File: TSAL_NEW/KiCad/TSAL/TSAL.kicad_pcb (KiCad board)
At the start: 2 copper layers, 74.8 x 40.6 mm, 34 parts, among them J1 HV INPUT, J2 HV GND, J3 Pin Storage, J4 Green_LED_Jp, J5 Conn_02x02_Counter_Clockwise, Q1 BSS84, Q2 BSS84, U1 LTV-817S, U2 LR8K4-G, U4 LM555

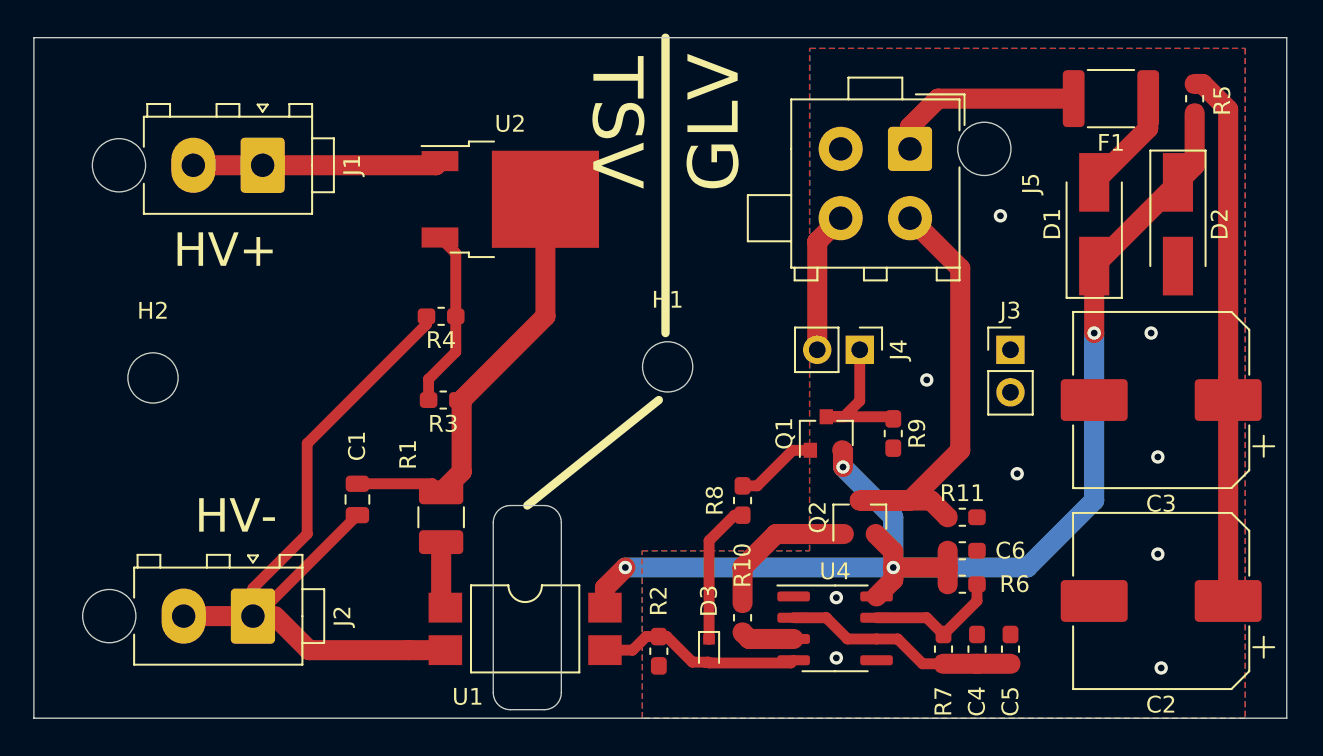
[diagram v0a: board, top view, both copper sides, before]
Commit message: TSAL Review complete
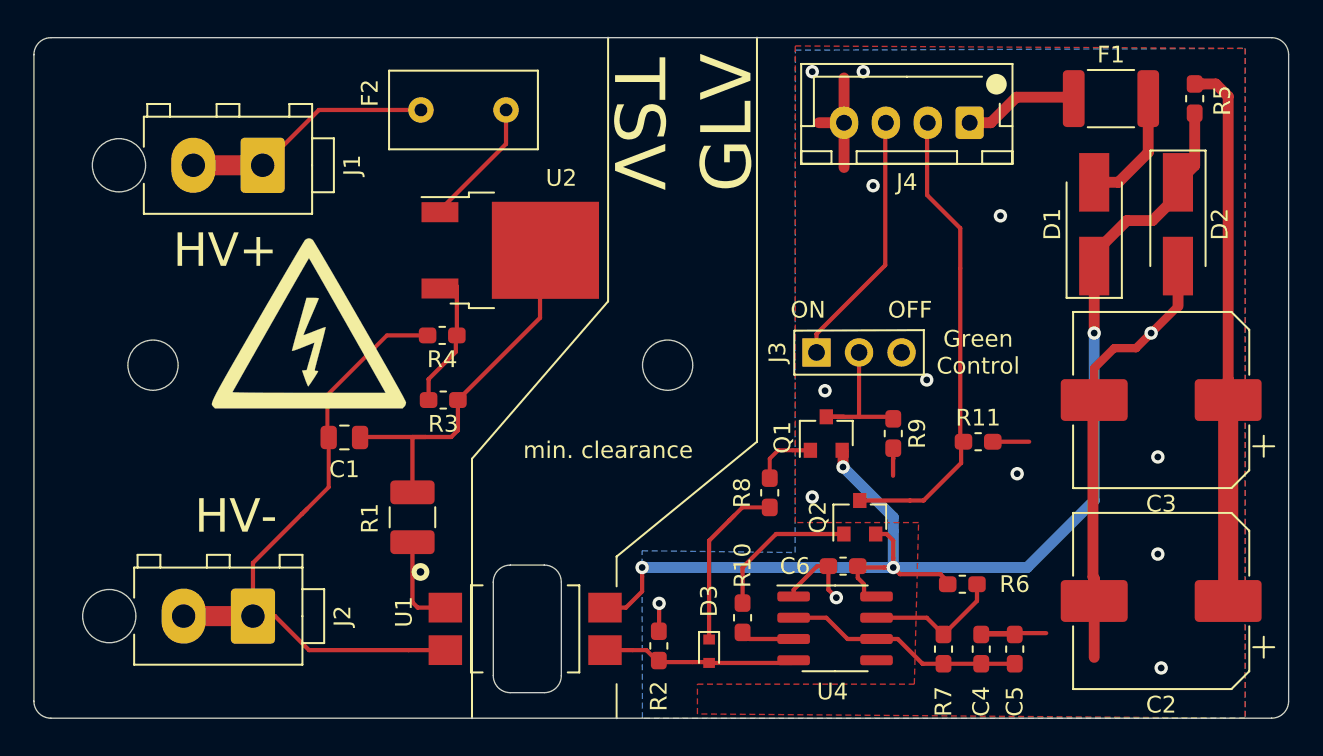
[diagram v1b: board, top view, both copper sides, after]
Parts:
- removed J5: Conn_02x02_Counter_Clockwise, Connector_TE-Connectivity:TE_MATE-N-LOK_1-770874-x_2x02_P4.14mm_Vertical
- added F2: Fuse, TSAL:PCC-1_2-R, F.Cu at (134.9, 90.7)
- added REF**: JUMPER_BLUE, TSAL:JUMPER_BLUE, F.Cu at (153.4, 105.2)
- added Ref**: Val**, TSAL:blinky, B.Cu at (166.9, 109.0)
- added Ref**: Val**, TSAL:zap, B.Cu at (125.5, 91.9)
- added Ref**: Val**, TSAL:zap, F.Cu at (128.0, 98.6)
- J1, J2: footprint Connector_TE-Connectivity:TE_MATE-N-LOK_1-770866-x_1x02_P4.14mm_Vertical -> TSAL:TE_MATE-N-LOK_1-770866-x_1x02_P4.14mm_Vertical
- J3: value Pin Storage -> Conn_01x03; footprint Connector_PinHeader_2.54mm:PinHeader_1x02_P2.54mm_Vertical -> Connector_PinHeader_2.54mm:PinHeader_1x03_P2.54mm_Vertical
- J4: value Green_LED_Jp -> Conn_01x04; footprint Connector_PinHeader_2.54mm:PinHeader_1x02_P2.54mm_Vertical -> TSAL:JST_XH_B4B-XH-AM_1x04_P2.50mm_Vertical
- moved J4 15.1 mm to (162.6, 91.4), turned to 180 degrees
- moved J3 11.6 mm to (153.4, 105.2), turned to 90 degrees
- moved C6 7.18 mm to (155.0, 117.9), turned to 180 degrees
- moved R11 4.61 mm to (163.1, 110.5)
- moved C1 3.78 mm to (125.2, 110.2), turned to 180 degrees
- moved U2 3.05 mm to (135.1, 99.1)
- moved R1 1.71 mm to (129.3, 115.0)
- moved R8 1.69 mm to (150.6, 113.5)
- moved R4 1.14 mm to (131.1, 104.1)
- moved H2 0.76 mm to (113.8, 105.9)
- moved R2 0.32 mm to (144.0, 122.7), turned to 90 degrees
- moved C4 0.25 mm to (163.3, 122.9)
- moved C5 0.25 mm to (165.3, 122.9)
- moved H1 0.10 mm to (144.5, 105.9)
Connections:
- net Net-(D1-Pad2) renamed /FUSE+
- net Net-(D3-Pad1) renamed /LGR_D
- net Net-(Q1-Pad1) renamed /LGR_G+
- net Net-(R1-Pad2) renamed /OPT+
- net Net-(R3-Pad2) renamed /ADJ
- J3 pad 1: Net-(J3-Pad1) -> /LED_GREEN+
- J3 pad 2: Net-(J3-Pad2) -> /LED_GREEN_OUT
- J4 pad 1: /LED_GREEN_OUT -> /GLV+
- J4 pad 2: /LED_GREEN+ -> /LED_RED+
- U2 pad 1: /HV+ -> /HV+F
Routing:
- net GND: track 0.00 -> 53.0 mm, vias 9 -> 14
- net GNDA: track 47.4 -> 39.9 mm
- net /HV+F: track 0.00 -> 7.42 mm
- net /LED_GREEN+: track 8.44 -> 15.4 mm
- net /GLV+: track 11.8 -> 6.73 mm
- net /ADJ: track 10.8 -> 7.58 mm
- net /LGR_D: track 8.53 -> 10.8 mm
- net /OPT+: track 4.01 -> 5.95 mm
- net /LGR_G+: track 4.93 -> 3.91 mm
- net /12V_CAP: track 32.0 -> 32.9 mm
- net /FUSE+: track 6.34 -> 7.26 mm
- net /HV_PRES: track 12.3 -> 11.7 mm
- net +12V: track 76.3 -> 76.8 mm
- net /LED_GREEN_OUT: track 9.04 -> 8.52 mm
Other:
- board size 74.8 x 40.6 mm -> 74.9 x 40.6 mm
- net class HIGH_CUR added: clearance 0.2, trace_width 0.5, via_dia 0.8, via_drill 0.4
- board text added: "GND GRN+ RED+ GLV+"
- board text added: "Green Control"
- board text added: "OFF"
- board text added: "ON"
- board text added: "min. clearance"
